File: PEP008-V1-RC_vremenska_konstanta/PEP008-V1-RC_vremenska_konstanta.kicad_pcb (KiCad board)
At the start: 2 copper layers, 45 x 45 mm, 19 parts, among them J1 Conn_01x01_Pin, J2 Screw_Terminal_01x02, J3 Conn_01x01_Pin, J4 Conn_01x01_Pin, J5 Conn_01x01_Pin, J6 Conn_01x03_Pin, J7 Conn_01x03_Pin, SW1 SW_SPDT, SW2 SW_SPDT

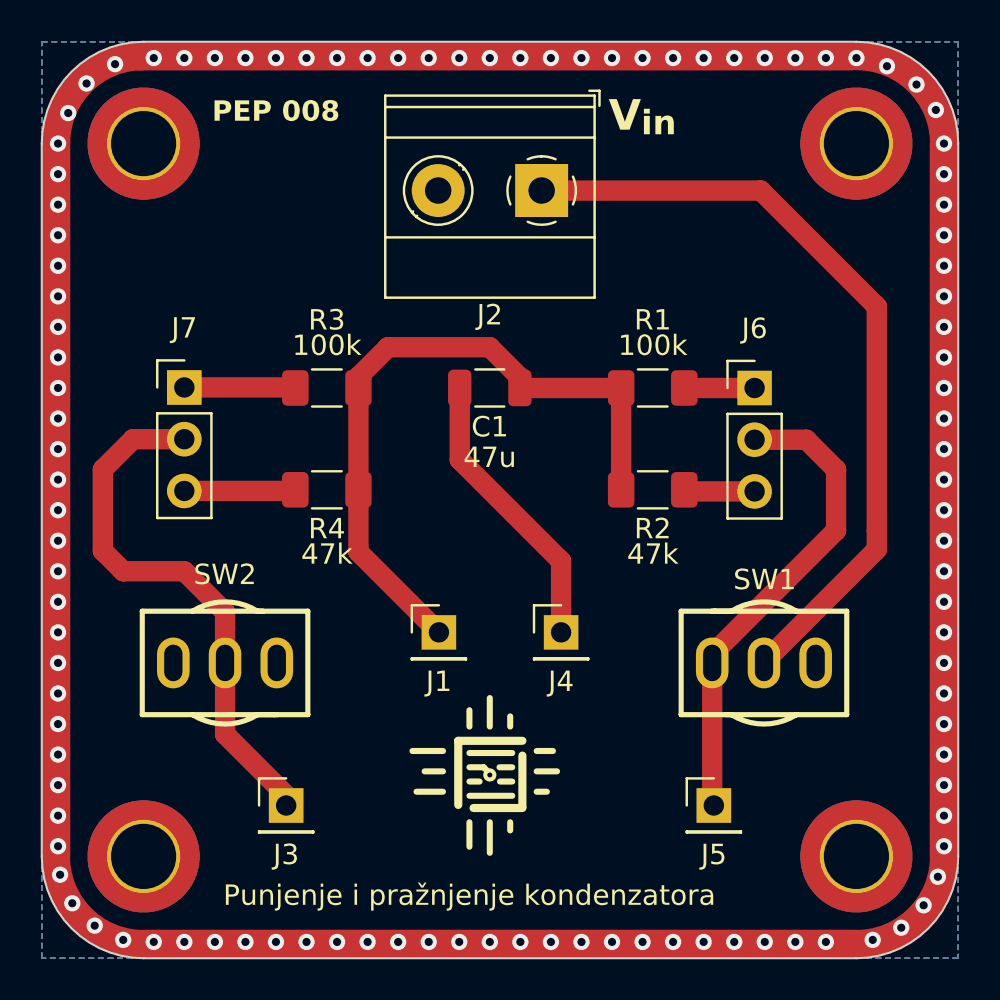
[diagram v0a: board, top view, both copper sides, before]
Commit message: PEP008 final commit, ready for production.
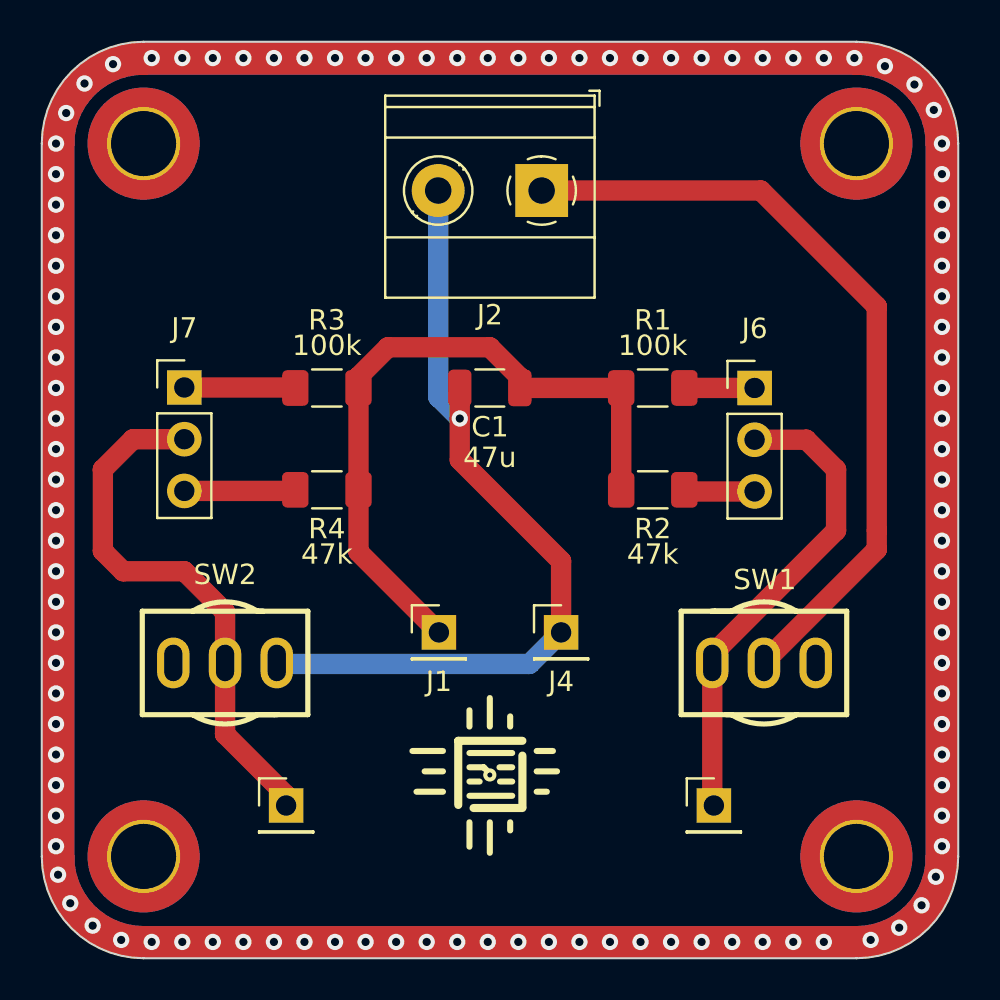
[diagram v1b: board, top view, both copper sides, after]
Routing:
- net 0: track 14.1 -> 40.3 mm, vias 109 -> 1
- net (no net): vias 0 -> 109
- removed copper zone on B.Cu, net 0
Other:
- board text removed: "PEP 008"
- board text removed: "Punjenje i pražnjenje kondenzatora"
- board text removed: "V_{in}"
